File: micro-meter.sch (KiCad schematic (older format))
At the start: 106 parts, among them U1 XC6206P332MR, U2 STM32F411CEU6

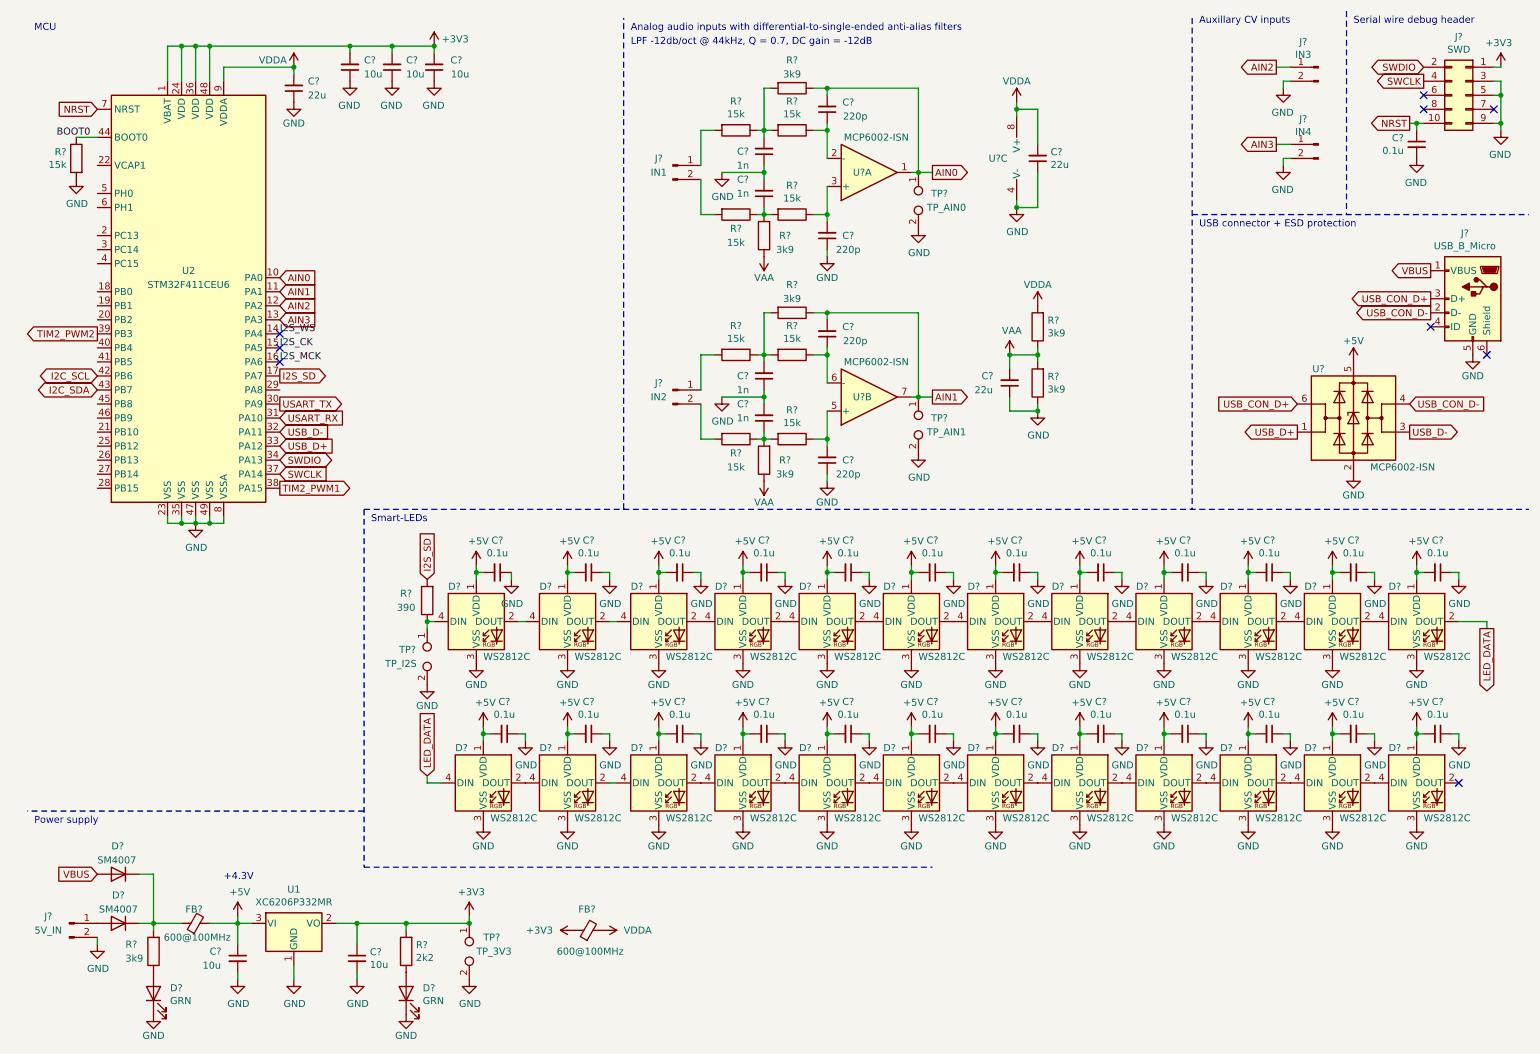
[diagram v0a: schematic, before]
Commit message: Cleanup schematics
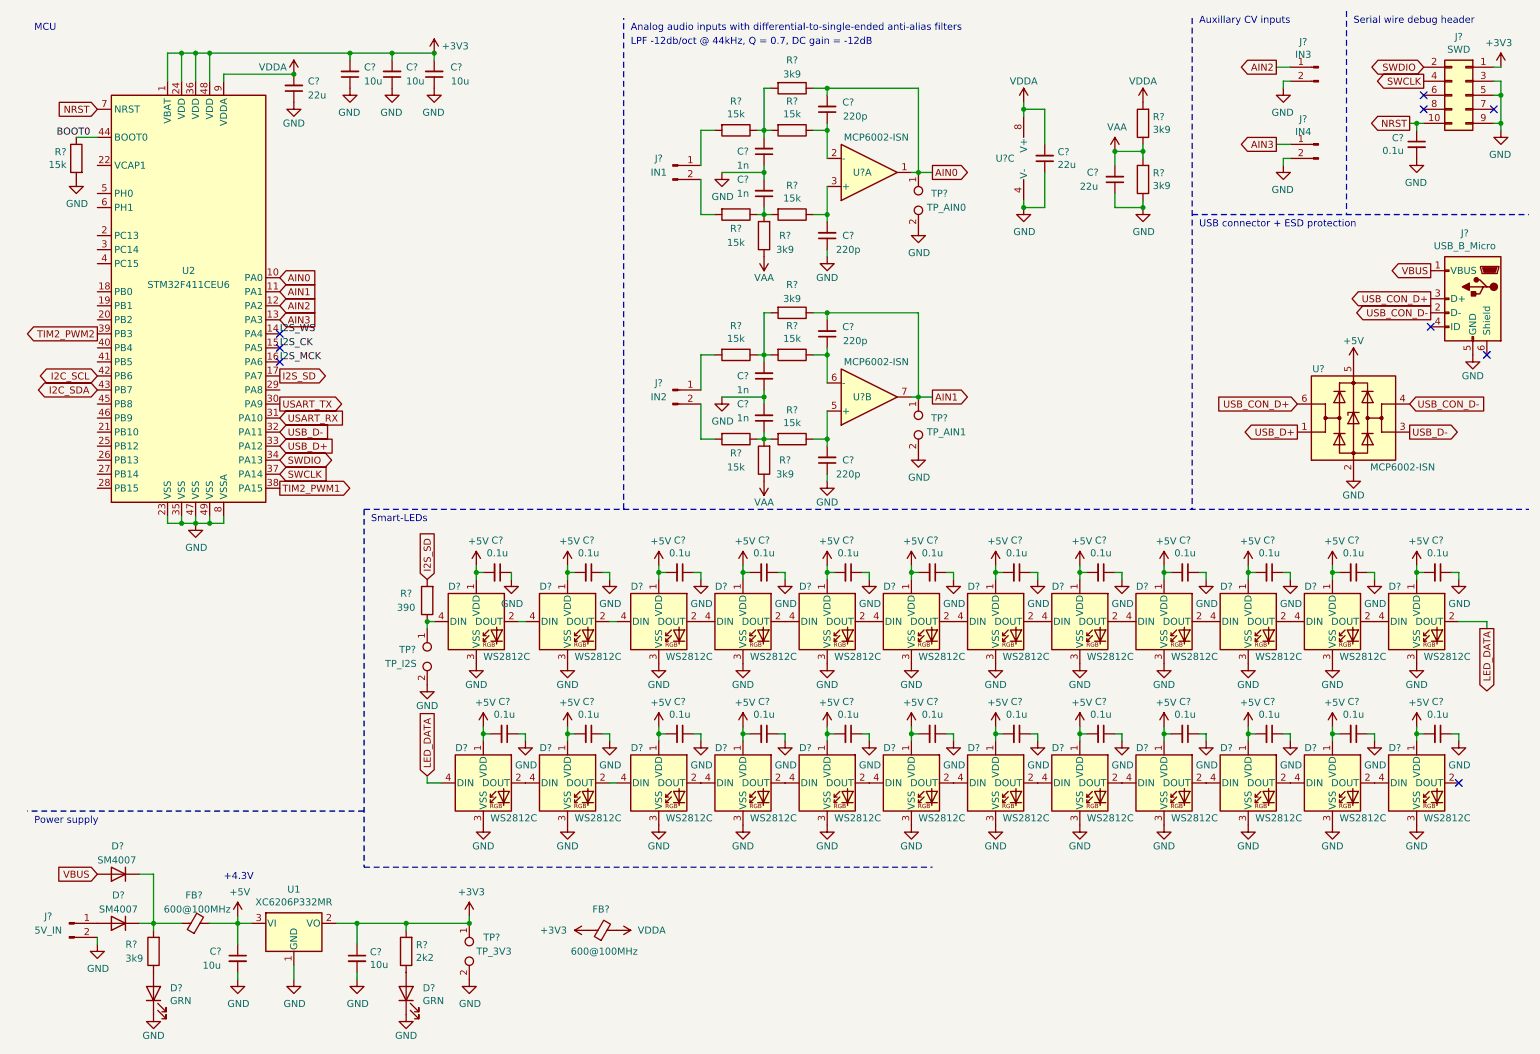
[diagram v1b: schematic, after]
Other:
- moved on the sheet: C?, FB?, R?, U?C
